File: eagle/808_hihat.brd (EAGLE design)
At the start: 100 x 80 mm, 127 parts, among them IC1 TL072P, IC2 TL072P, U4 4584N

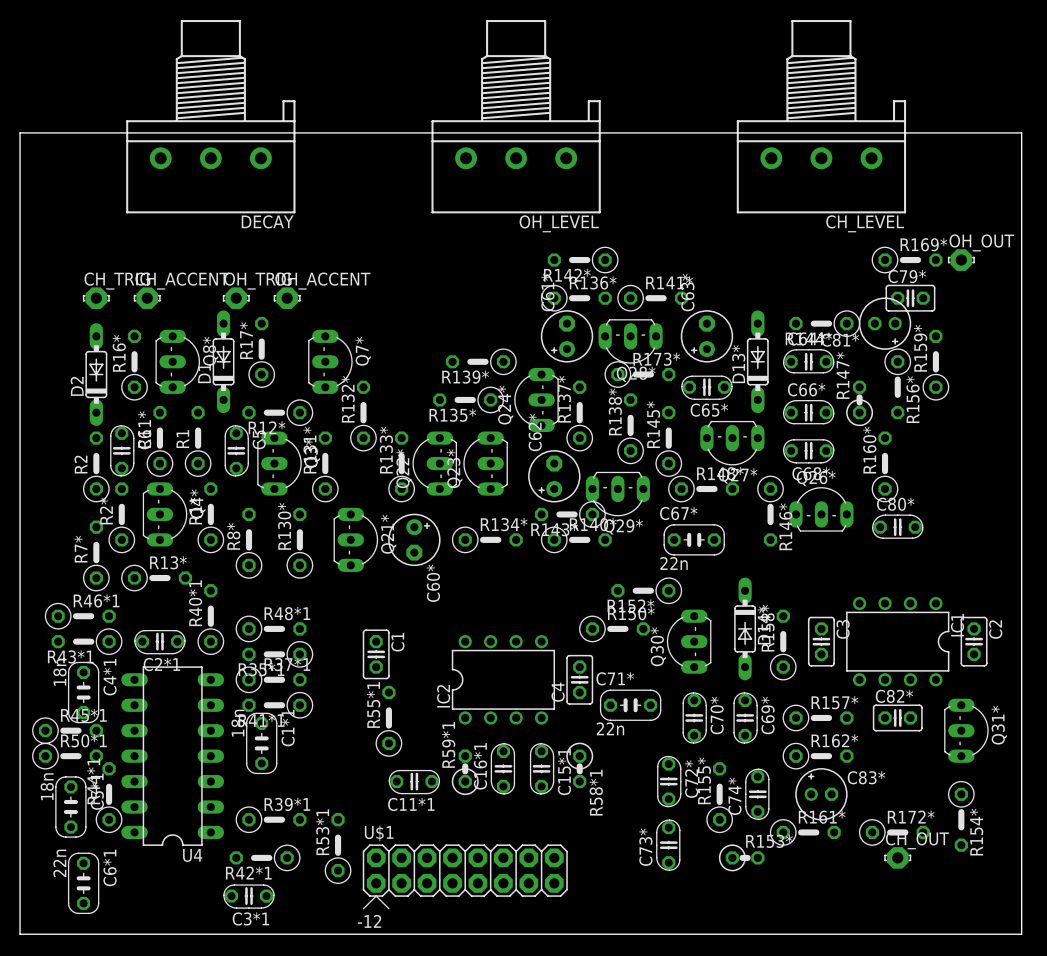
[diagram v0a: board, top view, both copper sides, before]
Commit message: baby steps
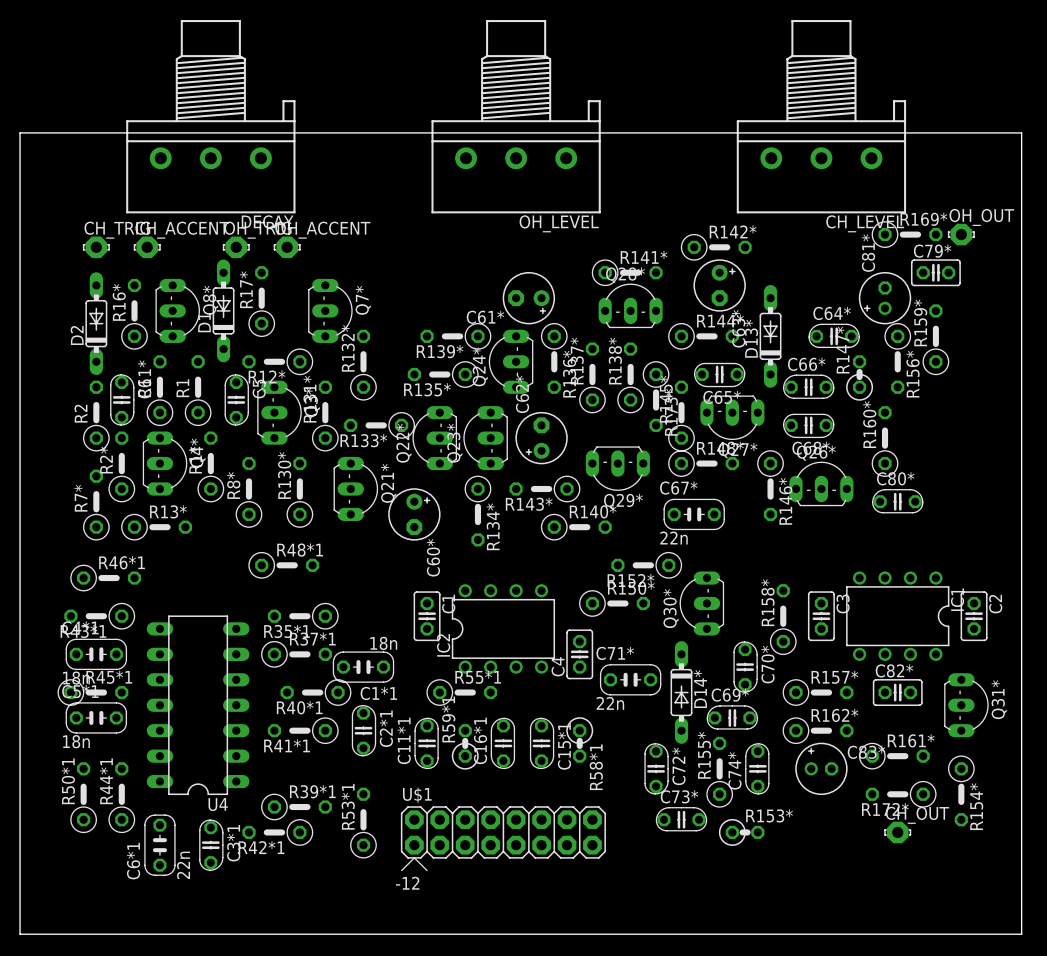
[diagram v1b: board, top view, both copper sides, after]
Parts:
- moved C2*1 22.2 mm to (34.3, 20.3), turned to 270 degrees
- moved R142* 14.0 mm to (69.8, 68.6), turned to 0 degrees
- moved C1*1 12.7 mm to (34.3, 26.7), turned to 180 degrees
- moved R40*1 12.7 mm to (29.2, 24.1), turned to 180 degrees
- moved R161* 11.7 mm to (87.6, 17.8)
- moved R144* 11.5 mm to (68.6, 59.7), turned to 0 degrees
- moved C5*1 9.25 mm to (7.62, 21.6), turned to 0 degrees
- moved D14* 8.98 mm to (66.0, 24.1)
- moved C6*1 8.52 mm to (14.0, 8.89), turned to 90 degrees
- moved R55*1 8.03 mm to (44.5, 24.1), turned to 0 degrees
- moved C70* 7.18 mm to (72.4, 26.7)
- moved R136* 6.84 mm to (53.3, 57.1), turned to 270 degrees
- moved R48*1 6.48 mm to (26.7, 36.8)
- moved C3*1 6.35 mm to (19.1, 8.89), turned to 270 degrees
- moved C1 6.35 mm to (40.6, 31.8)
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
